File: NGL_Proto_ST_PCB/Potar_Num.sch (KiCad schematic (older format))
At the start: 2 parts, among them U10 10K, U11 AD5270BRMZ-20-RL7

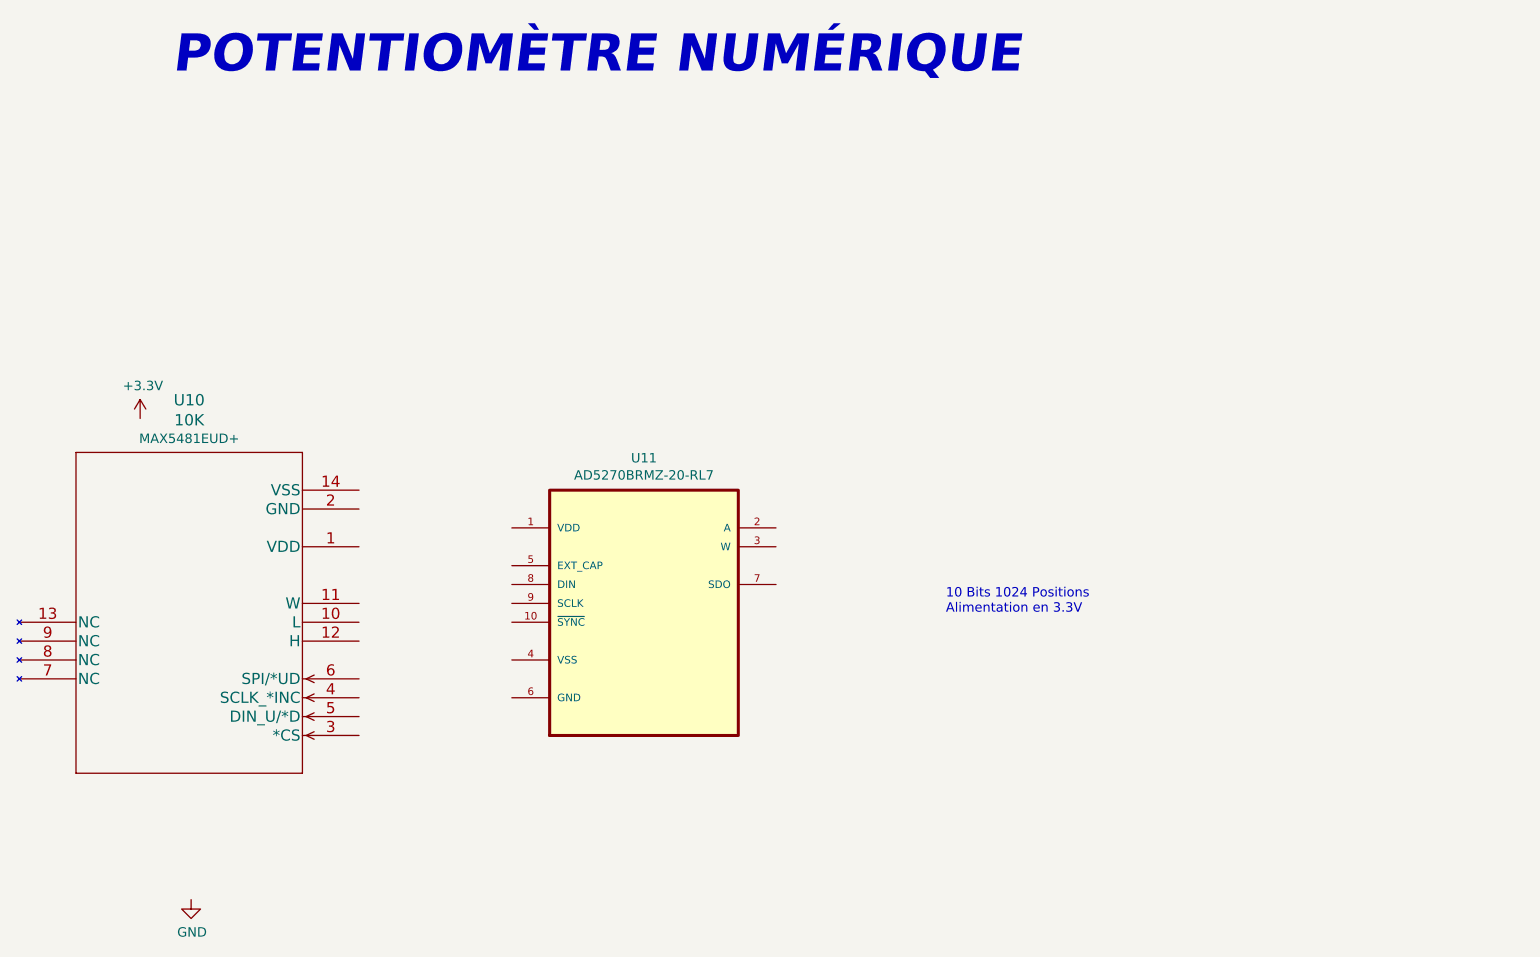
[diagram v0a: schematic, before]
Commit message: amélioration
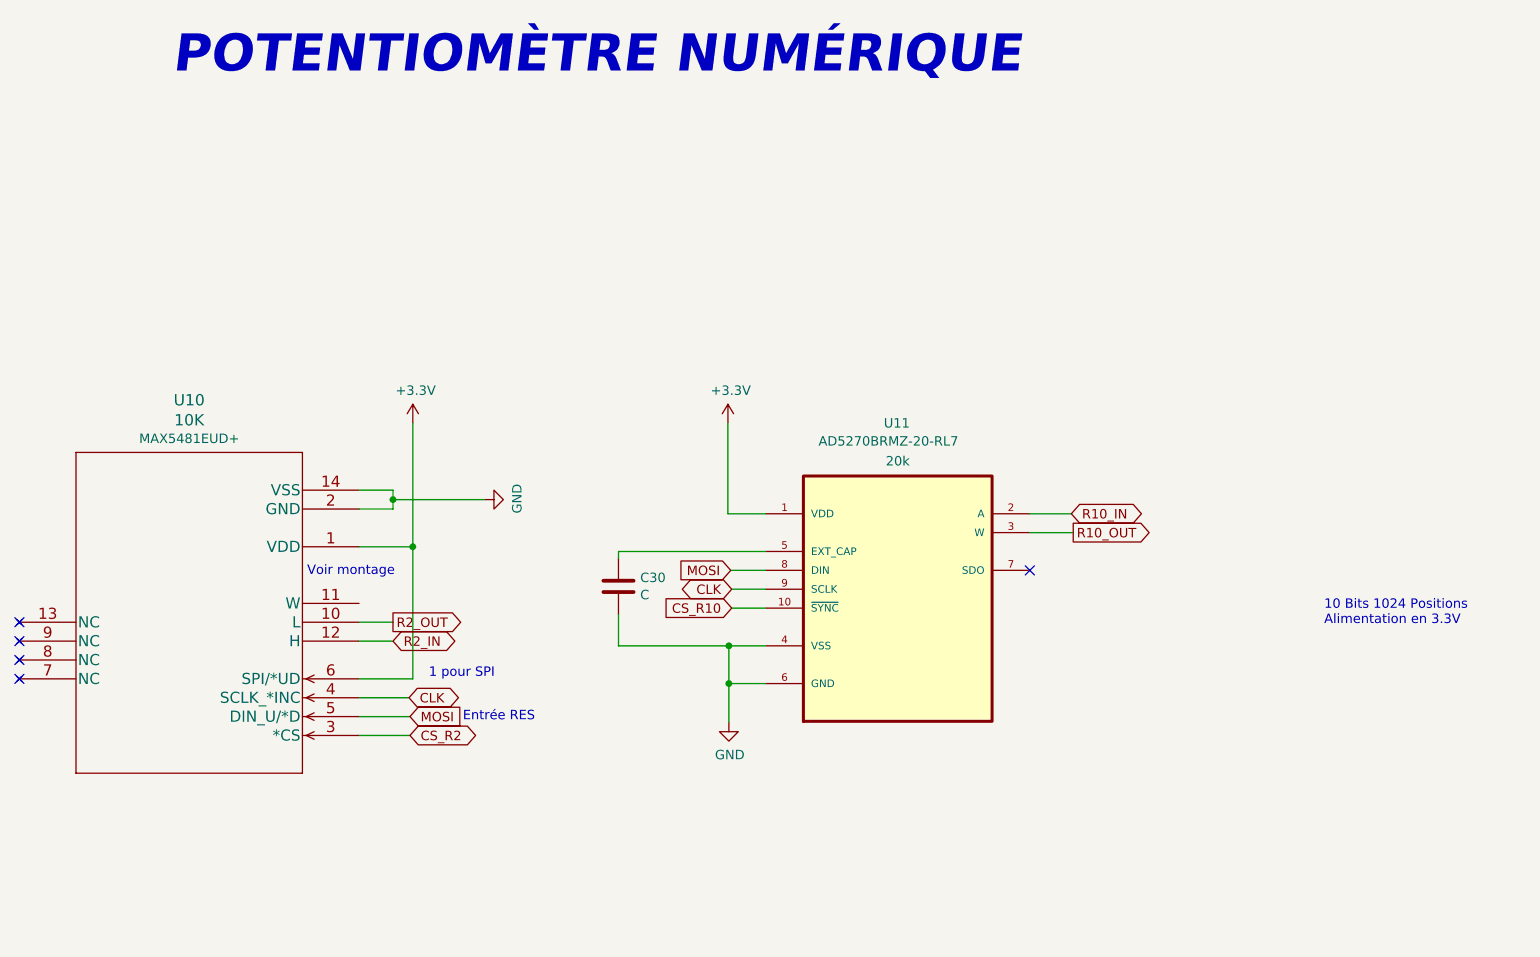
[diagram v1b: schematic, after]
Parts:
- added C30: C, Capacitor_SMD:C_0805_2012Metric, symbol Device:C
- U11: value AD5270BRMZ-20-RL7 -> 20k; OC_FARNELL - -> (none); PACKAGE MSOP-10 -> (none)
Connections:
- net +3V3: now also U10.1 (VDD), U10.6 (SPI/*UD), U11.1 (VDD)
- net GND: now also U10.14 (VSS), U10.2 (GND), U11.4 (VSS), U11.6 (GND), C30.2
- net R2_OUT: now reaches U10.10 (L)
- net R2_IN: now reaches U10.12 (H)
- net CS_R2: now reaches U10.3 (*CS)
- net CLK: now reaches U10.4 (SCLK_*INC)
- net CLK: now also U11.9 (SCLK)
- net MOSI: now reaches U10.5 (DIN_U/*D)
- net MOSI: now also U11.8 (DIN)
- net CS_R10: now reaches U11.10 (~SYNC)
- net R10_IN: now reaches U11.2 (A)
- net R10_OUT: now reaches U11.3 (W)
- net at U11.5 (EXT_CAP): now also C30.1
- no-connect marks 0 -> 5
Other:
- note added: "1 pour SPI"
- note added: "Entrée RES"
- note added: "Voir montage"
- moved on the sheet: U11
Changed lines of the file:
@@
 $EndDescr
+$Comp
+L power:+3.3V #PWR015
+U 1 1 62947A80
+P 6665 3645
+F 0 "#PWR015" H 6665 3495 50  0001 C CNN
+F 1 "+3.3V" H 6680 3818 50  0000 C CNN
+F 2 "" H 6665 3645 50  0001 C CNN
+F 3 "" H 6665 3645 50  0001 C CNN
+	1    6665 3645
+	1    0    0    -1
+$EndComp
+$Comp
+L power:GND #PWR016
+U 1 1 629496F5
+P 5375 4050
+F 0 "#PWR016" H 5375 3800 50  0001 C CNN
+F 1 "GND" H 5380 3877 50  0000 C CNN
+F 2 "" H 5375 4050 50  0001 C CNN
+F 3 "" H 5375 4050 50  0001 C CNN
+	1    5375 4050
+	0    -1   -1   0
+$EndComp
+Text Notes 3720 1810 0    197  Italic 39
+POTENTIOMÈTRE NUMÉRIQUE
+Text Notes 9825 4720 0    50   ~ 0
+10 Bits 1024 Positions\nAlimentation en 3.3V
+$Comp
+L AD5270BRMZ-20-RL7:AD5270BRMZ-20-RL7 U11
+U 1 1 6295B510
+P 7565 4425
+F 0 "U11" H 7560 5205 50  0000 C CNN
+F 1 "20k" H 7565 5004 50  0000 C CNN
+F 2 "Lib_NGL_ST:SOP50P490X110-10N" H 7565 4425 50  0001 L BNN
+F 3 "https://www.analog.com/media/en/technical-documentation/data-sheets/AD5270_5271.pdf" H 7565 4425 50  0001 L BNN
+F 4 "Analog Devices" H 7565 4425 50  0001 L BNN "SUPPLIER"
+F 5 "52R8111" H 7565 4425 50  0001 L BNN "OC_NEWARK"
+F 6 "AD5270BRMZ-20-RL7" H 7145 5080 50  0000 L BNN "MPN"
+	1    7565 4425
+	1    0    0    -1
+$EndComp
+Text GLabel 4975 5100 2    50   BiDi ~ 0
+CLK
+Text GLabel 4980 5300 2    50   BiDi ~ 0
+CS_R2
+Text GLabel 6680 4425 0    50   Input ~ 0
+MOSI
+Text Notes 5260 5230 0    50   ~ 0
+Entrée RES
+Text GLabel 4890 4800 2    50   BiDi ~ 0
+R2_IN
+Text GLabel 4890 4700 2    50   Output ~ 0
+R2_OUT
+Text GLabel 8485 4125 2    50   BiDi ~ 0
+R10_IN
+Text GLabel 8495 4225 2    50   Output ~ 0
+R10_OUT
+Text GLabel 6685 4525 0    50   BiDi ~ 0
+CLK
+$Comp
+L power:GND #PWR042
+U 1 1 629B014D
+P 6670 5230
+F 0 "#PWR042" H 6670 4980 50  0001 C CNN
+F 1 "GND" H 6675 5057 50  0000 C CNN
+F 2 "" H 6670 5230 50  0001 C CNN
+F 3 "" H 6670 5230 50  0001 C CNN
+	1    6670 5230
+	1    0    0    -1
+$EndComp
+Text GLabel 4980 5200 2    50   Input ~ 0
+MOSI
+NoConn ~ 8265 4425
+Wire Wire Line
+	4980 5200 4710 5200
+Wire Wire Line
+	4710 5100 4975 5100
+Wire Wire Line
+	4890 4800 4710 4800
+Wire Wire Line
+	4890 4700 4710 4700
+Text Notes 4435 4460 0    50   ~ 0
+Voir montage
+$Comp
+L power:+3.3V #PWR040
+U 1 1 629B80B0
+P 4995 3645
+F 0 "#PWR040" H 4995 3495 50  0001 C CNN
+F 1 "+3.3V" H 5010 3818 50  0000 C CNN
+F 2 "" H 4995 3645 50  0001 C CNN
+F 3 "" H 4995 3645 50  0001 C CNN
+	1    4995 3645
+	1    0    0    -1
+$EndComp
+Wire Wire Line
+	4710 4000 4890 4000
+Wire Wire Line
+	4890 4000 4890 4050
+Wire Wire Line
+	4890 4050 5375 4050
+Wire Wire Line
+	4710 4100 4890 4100
+Wire Wire Line
+	4890 4100 4890 4050
+Connection ~ 4890 4050
+Wire Wire Line
+	4995 3645 4995 4300
+Wire Wire Line
+	4995 4300 4710 4300
+Wire Wire Line
+	6665 3645 6665 4125
+Wire Wire Line
+	6665 4125 6865 4125
+Wire Wire Line
+	8485 4125 8265 4125
+Wire Wire Line
+	8495 4225 8265 4225
+Wire Wire Line
+	6865 4425 6680 4425
+Wire Wire Line
+	6865 4525 6685 4525
+Wire Wire Line
+	6670 5025 6865 5025
+Wire Wire Line
+	6865 4825 6670 4825
+Wire Wire Line
+	6670 4825 6670 5025
+Connection ~ 6670 5025
+Wire Wire Line
+	6670 5025 6670 5230
+NoConn ~ 2910 5000
+NoConn ~ 2910 4900
+NoConn ~ 2910 4800
+NoConn ~ 2910 4700
 $Comp
 L max5481eud&plus_T:max5481eud+T U10
@@
 	-1   0    0    1
 $EndComp
+Text GLabel 6685 4625 0    50   Input ~ 0
+CS_R10
+Wire Wire Line
+	6865 4625 6685 4625
 $Comp
-L power:+3.3V #PWR015
-U 1 1 62947A80
-P 3550 3620
-F 0 "#PWR015" H 3550 3470 50  0001 C CNN
-F 1 "+3.3V" H 3565 3793 50  0000 C CNN
-F 2 "" H 3550 3620 50  0001 C CNN
-F 3 "" H 3550 3620 50  0001 C CNN
-	1    3550 3620
+L Device:C C30
+U 1 1 629BEC75
+P 6085 4510
+F 0 "C30" H 6200 4556 50  0000 L CNN
+F 1 "C" H 6200 4465 50  0000 L CNN
+F 2 "Capacitor_SMD:C_0805_2012Metric" H 6123 4360 50  0001 C CNN
+F 3 "~" H 6085 4510 50  0001 C CNN
+	1    6085 4510
 	1    0    0    -1
 $EndComp
-$Comp
-L power:GND #PWR016
-U 1 1 629496F5
-P 3820 6170
-F 0 "#PWR016" H 3820 5920 50  0001 C CNN
-F 1 "GND" H 3825 5997 50  0000 C CNN
-F 2 "" H 3820 6170 50  0001 C CNN
-F 3 "" H 3820 6170 50  0001 C CNN
-	1    3820 6170
-	1    0    0    -1
-$EndComp
-Text Notes 3720 1810 0    197  Italic 39
-POTENTIOMÈTRE NUMÉRIQUE
-Text Notes 7820 4660 0    50   ~ 0
-10 Bits 1024 Positions\nAlimentation en 3.3V
-$Comp
-L AD5270BRMZ-20-RL7:AD5270BRMZ-20-RL7 U11
-U 1 1 6295B510
-P 6220 4500
-F 0 "U11" H 6220 5170 50  0000 C CNN
-F 1 "AD5270BRMZ-20-RL7" H 6220 5079 50  0000 C CNN
-F 2 "Lib_NGL_ST:SOP50P490X110-10N" H 6220 4500 50  0001 L BNN
-F 3 "https://www.analog.com/media/en/technical-documentation/data-sheets/AD5270_5271.pdf" H 6220 4500 50  0001 L BNN
-F 4 "Analog Devices" H 6220 4500 50  0001 L BNN "SUPPLIER"
-F 5 "52R8111" H 6220 4500 50  0001 L BNN "OC_NEWARK"
-F 6 "MSOP-10" H 6220 4500 50  0001 L BNN "PACKAGE"
-F 7 "AD5270BRMZ-20-RL7" H 6220 4500 50  0001 L BNN "MPN"
-F 8 "-" H 6220 4500 50  0001 L BNN "OC_FARNELL"
-	1    6220 4500
-	1    0    0    -1
-$EndComp
+Wire Wire Line
+	6865 4325 6085 4325
+Wire Wire Line
+	6085 4325 6085 4360
+Wire Wire Line
+	6085 4660 6085 4825
+Wire Wire Line
+	6085 4825 6670 4825
+Connection ~ 6670 4825
+Wire Wire Line
+	4980 5300 4710 5300
+Wire Wire Line
+	4995 4300 4995 5000
+Wire Wire Line
+	4995 5000 4710 5000
+Connection ~ 4995 4300
+Text Notes 5080 5000 0    50   ~ 0
+1 pour SPI
 $EndSCHEMATC
